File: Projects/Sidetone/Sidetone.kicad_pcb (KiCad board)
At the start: 2 copper layers, 90.6 x 92 mm, 54 parts, among them Q1 2N3904, Q2 2N3904, Q3 2N3904, SW1 morse key, SW2 On/off, U1 4N35, U2 LM324, U3 LM386

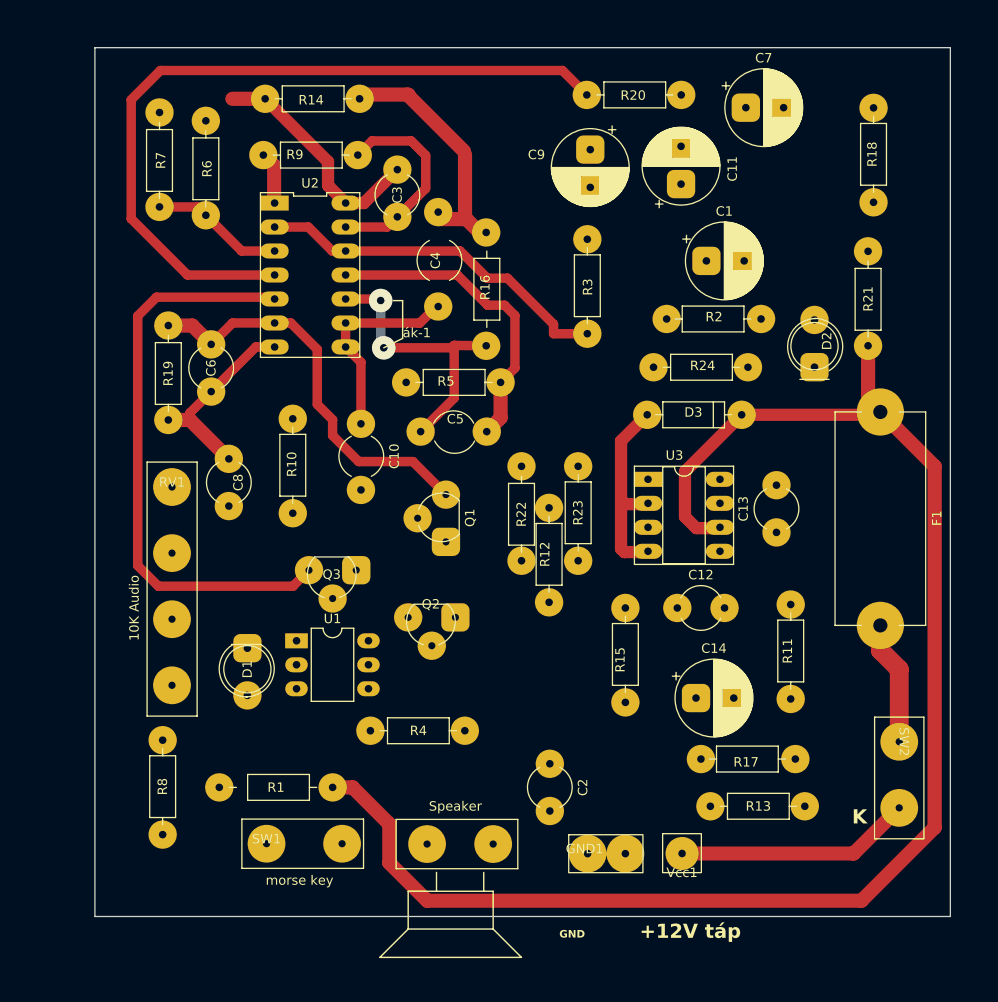
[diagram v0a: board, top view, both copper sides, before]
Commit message: 20240223
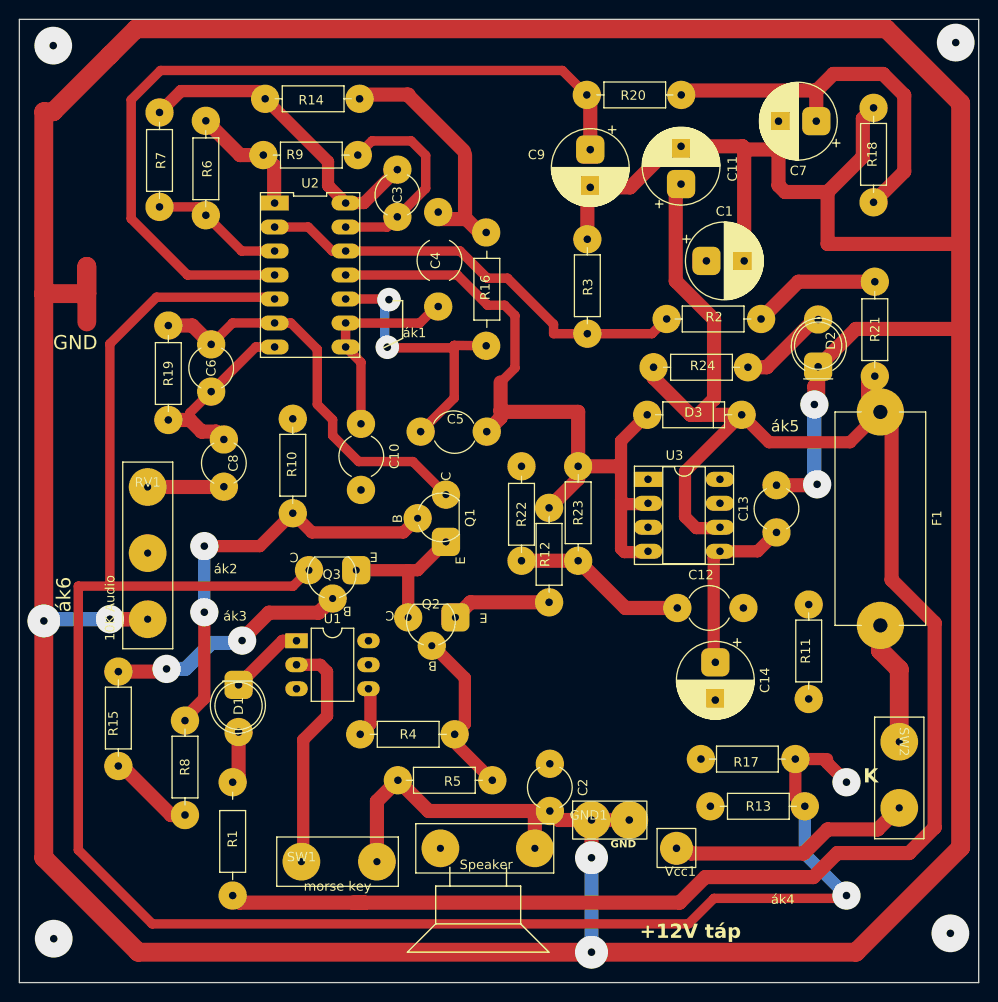
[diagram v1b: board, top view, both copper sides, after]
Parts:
- moved R15 54.1 mm to (101.9, 124.3)
- moved R5 37.3 mm to (137.2, 123.4), turned to 180 degrees
- moved C7 7.60 mm to (175.8, 56.0), turned to 180 degrees
- moved 4-8ohm1 5.61 mm to (136.0, 133.0), turned to 0 degrees
- moved C14 4.30 mm to (165.1, 113.3), turned to -90 degrees
- moved SW1 4.15 mm to (121.3, 134.4)
- moved D1 3.99 mm to (114.6, 115.7)
- moved GND1 3.59 mm to (152.0, 130.0)
- moved R21 3.30 mm to (182.0, 73.0)
- moved R8 3.14 mm to (109.0, 129.5)
- moved RV1 2.58 mm to (105.0, 94.7)
- moved C8 2.12 mm to (113.1, 89.7)
- moved R11 1.91 mm to (175.0, 117.2)
- moved R1 1.51 mm to (114.0, 126.0), turned to -90 degrees
- moved R4 1.14 mm to (127.5, 120.9)
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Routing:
- net GNDD: track 55.2 -> 644.8 mm, vias 0 -> 6
- net Net-(Q3-C): track 61.6 -> 210.5 mm, vias 0 -> 2
- net Net-(Q1-B): track 0.00 -> 44.8 mm, vias 0 -> 2
- net Net-(D3-K): track 161.0 -> 204.4 mm
- net Net-(C7-Pad1): track 0.00 -> 41.4 mm
- net Net-(Q3-B): track 0.00 -> 26.8 mm, vias 0 -> 2
- net Net-(SW1A-A): track 0.00 -> 24.8 mm
- net Net-(C13-Pad1): track 0.00 -> 18.9 mm
- net Net-(C12-Pad1): track 0.00 -> 18.6 mm
- net Net-(U2E-V+): track 101.6 -> 119.8 mm
- net Net-(Q2-B): track 0.00 -> 17.9 mm
- net Net-(Q1-E): track 0.00 -> 15.7 mm
- net Net-(Q2-E): track 0.00 -> 10.6 mm
- net Net-(D2-A): track 0.00 -> 9.53 mm
- net Net-(R15-Pad1): track 0.00 -> 9.20 mm
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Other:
- board size 90.6 x 92 mm -> 101.6 x 102 mm
- board text added: "ák1"
- board text added: "ák2"
- board text added: "ák3"
- board text added: "ák4"
- board text added: "ák5"
- board text added: "ák6"
- board text removed: "ák-1"
